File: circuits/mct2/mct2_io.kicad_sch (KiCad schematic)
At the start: 198 parts

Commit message: Aug 21, 2024 1
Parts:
- removed R? (x2): 10K, symbol Device:R_Small
- added L? (x2): 80@100MHz, symbol Device:L_Ferrite_Small
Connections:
- net M2E_3V3: now also L?.1
- net M2M_3V3: now also L?.1
- net HDMI_5V: now reaches C?.1, C?.2, L?.2, R?.1, U?.10 (VCC5V)
- net M2E_WDISABLE2: now reaches J?.54 (~{W_DISABLE2})
- net M2E_WDISABLE1: now reaches J?.56 (~{W_DISABLE1})
- net OLED_RES renamed OLED_RST
- new net M2_3V3: L?.2, L?.2
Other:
- note added: "July 4, 2024 - August 21, 2024"
- note removed: "July 4, 2024 - August 19, 2024"
- moved on the sheet: C?, D?, J?, J?A, J?B, JP?, L?, NT?, R?, T?, U?, Y?

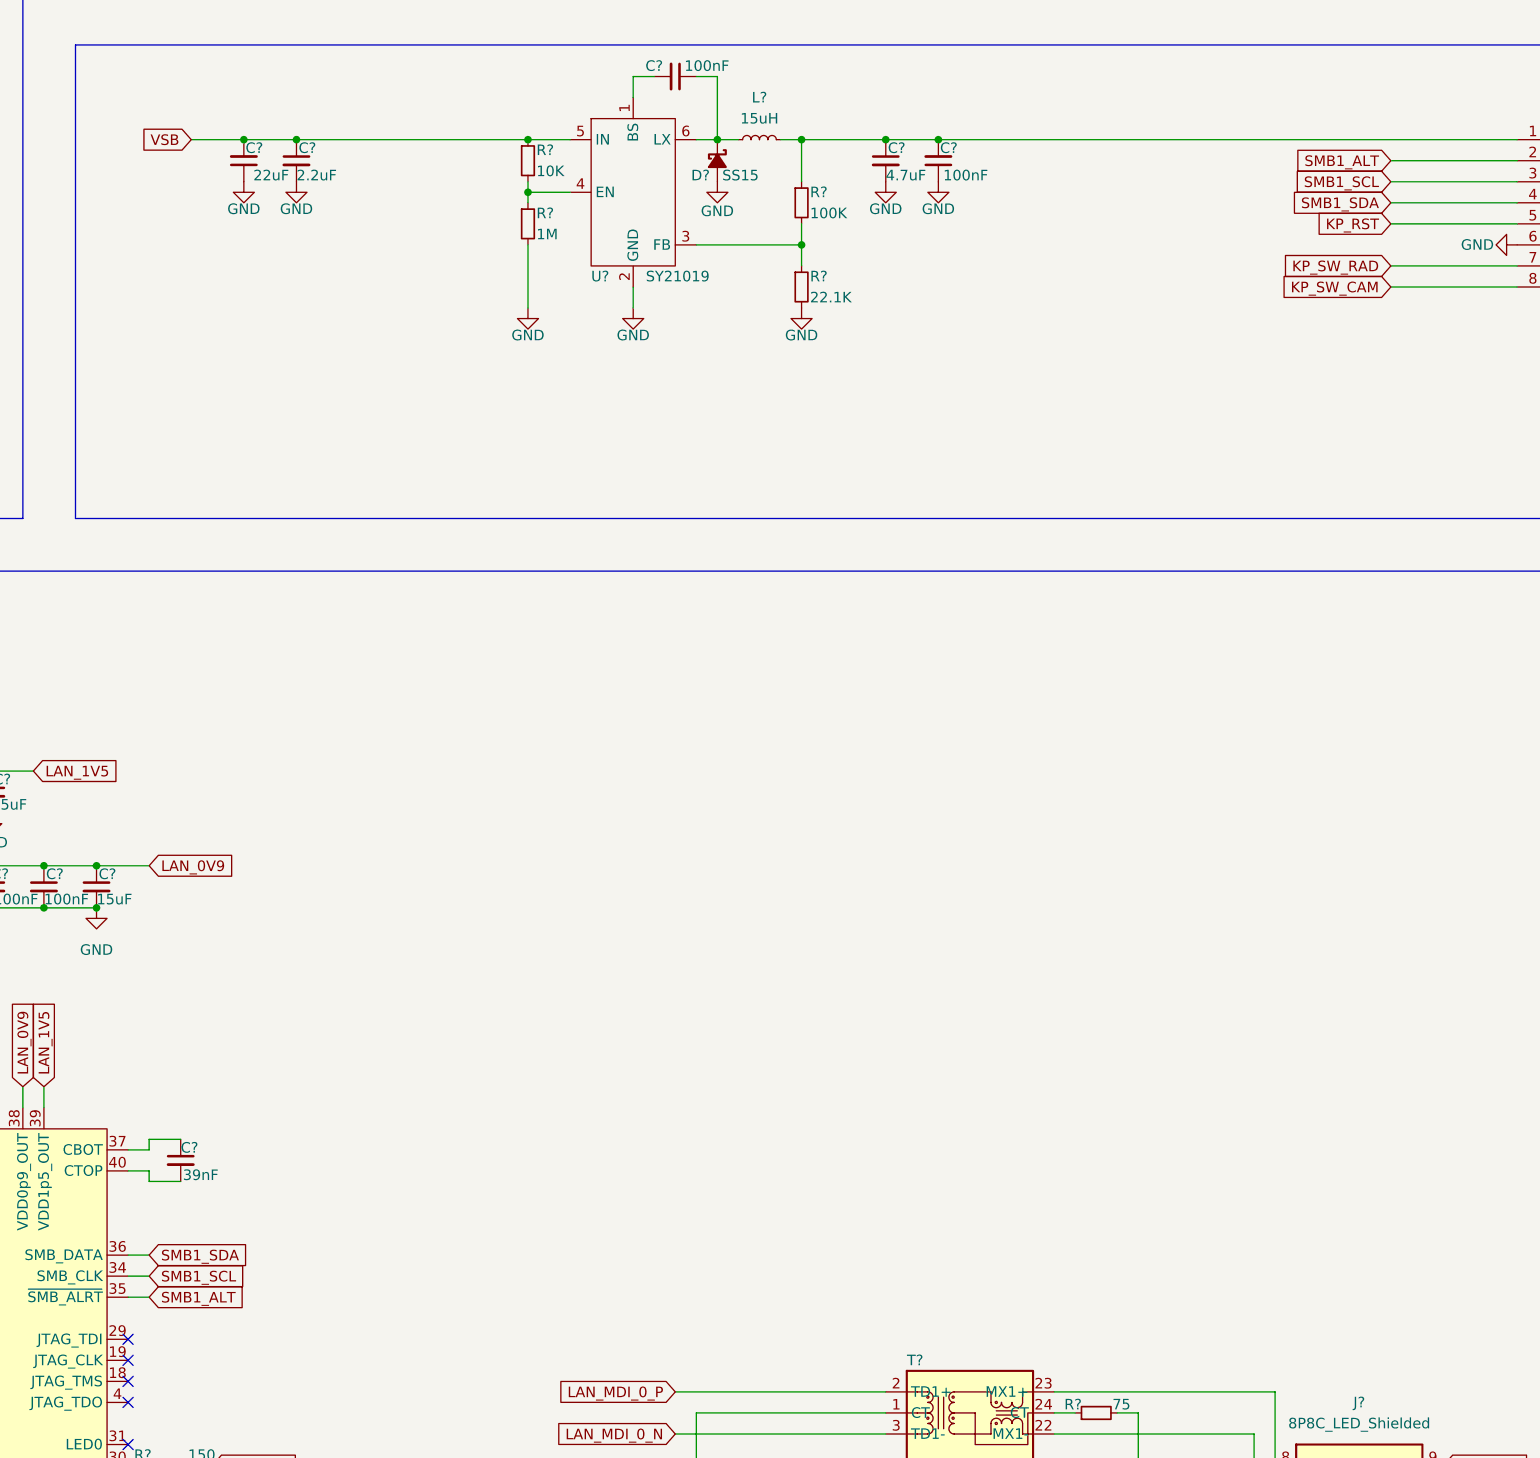
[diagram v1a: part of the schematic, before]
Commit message: Aug 22, 2024 1
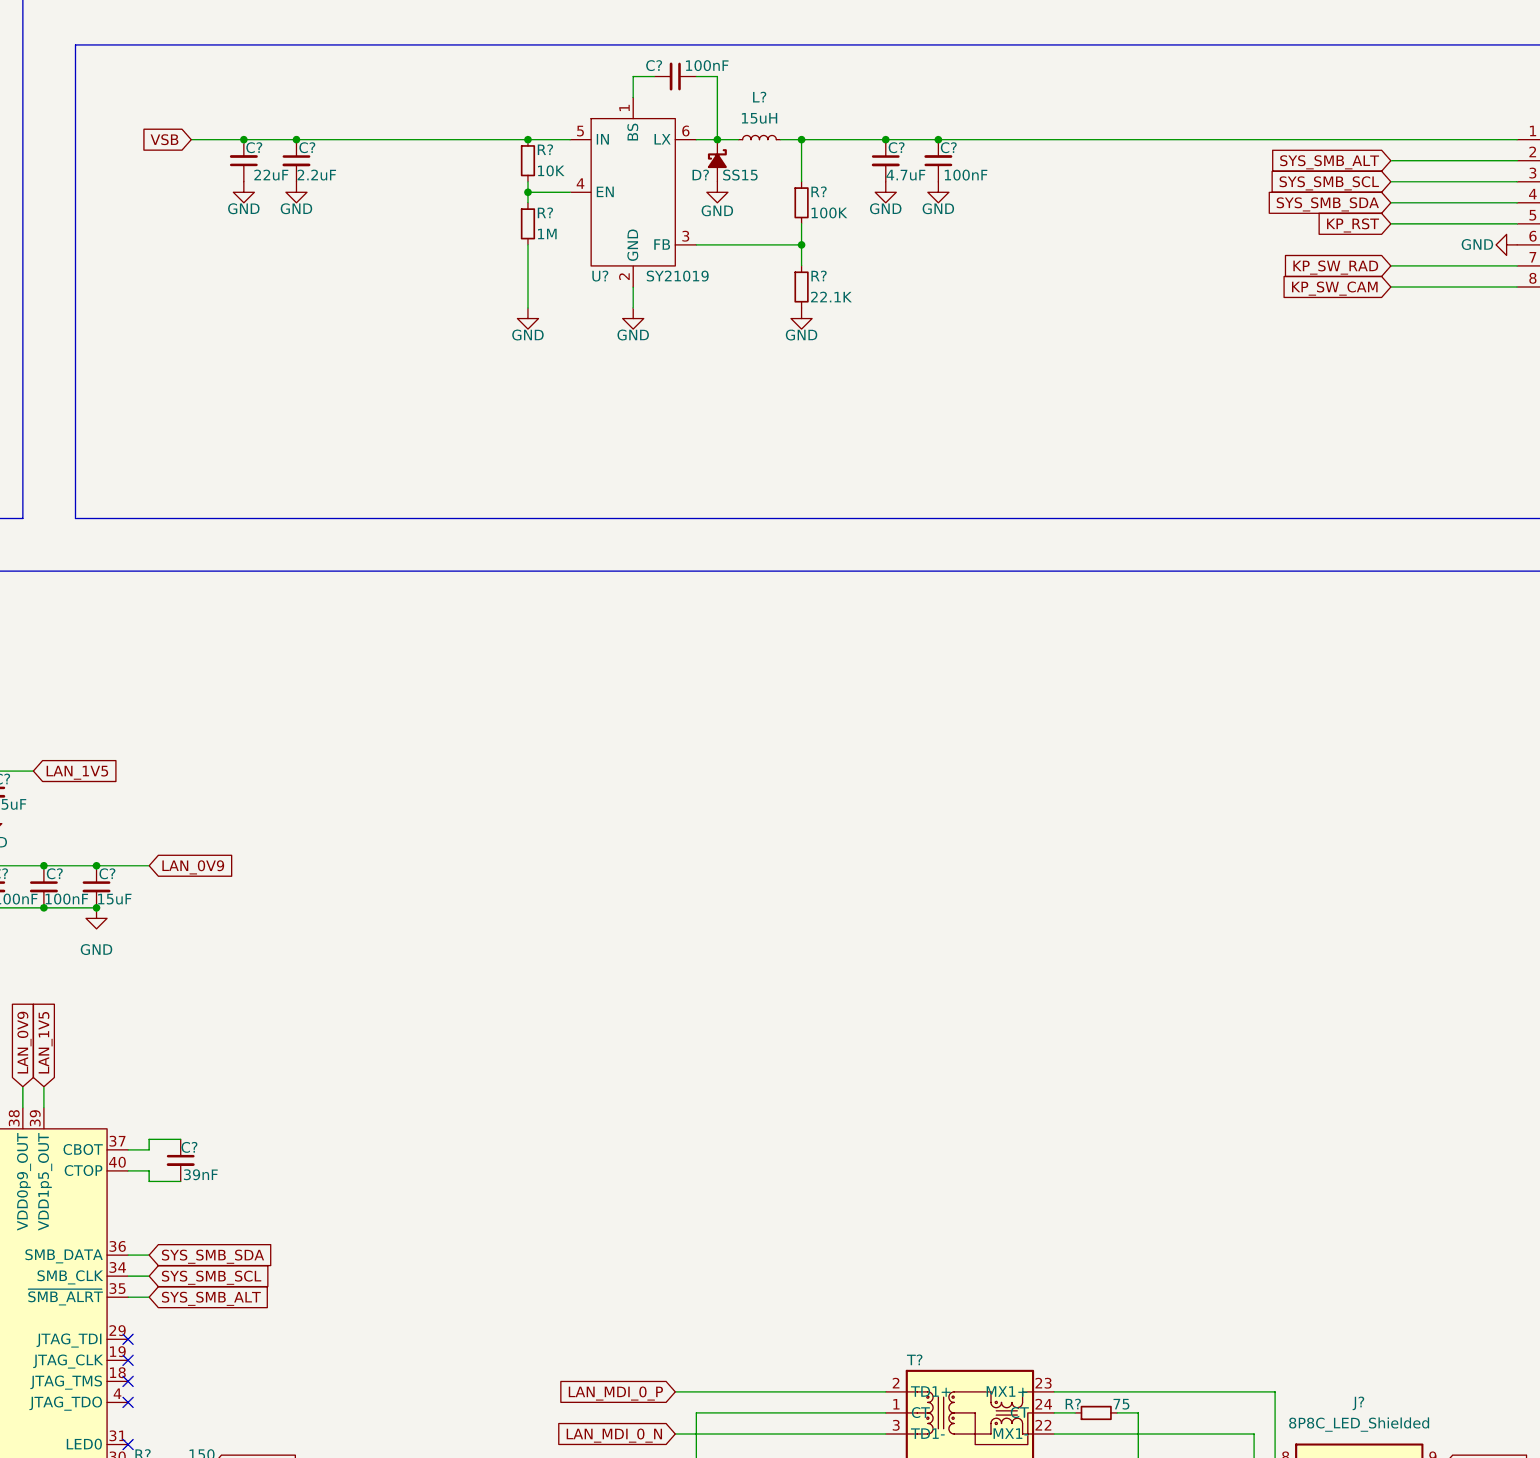
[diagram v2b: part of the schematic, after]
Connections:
- net SMB1_ALT renamed SYS_SMB_ALT
- net SMB1_SCL renamed SYS_SMB_SCL
- net SMB1_SDA renamed SYS_SMB_SDA
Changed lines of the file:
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@@
 		)
 	)
-	(global_label "SMB1_SCL"
+	(global_label "SYS_SMB_SCL"
 		(shape input)
 		(at 1131.57 321.31 180)
@@
 		)
 	)
-	(global_label "SMB1_SCL"
+	(global_label "SYS_SMB_SCL"
 		(shape input)
 		(at 981.71 453.39 0)
@@
 		)
 	)
-	(global_label "SMB1_ALT"
+	(global_label "SYS_SMB_ALT"
 		(shape input)
 		(at 981.71 455.93 0)
@@
 		)
 	)
-	(global_label "SMB1_SDA"
+	(global_label "SYS_SMB_SDA"
 		(shape input)
 		(at 981.71 450.85 0)
@@
 		)
 	)
-	(global_label "SMB1_ALT"
+	(global_label "SYS_SMB_ALT"
 		(shape input)
 		(at 1131.57 318.77 180)
@@
 		)
 	)
-	(global_label "SMB1_SDA"
+	(global_label "SYS_SMB_SDA"
 		(shape input)
 		(at 1131.57 323.85 180)
@@
 	)
 	(symbol
-		(lib_name "mediacow:TPD4EUSB30")
 		(lib_id "mediacow:TPD4EUSB30")
 		(at 1126.49 148.59 0)
@@
 	)
 	(symbol
-		(lib_name "mediacow:TPD4EUSB30")
 		(lib_id "mediacow:TPD4EUSB30")
 		(at 1126.49 82.55 0)
